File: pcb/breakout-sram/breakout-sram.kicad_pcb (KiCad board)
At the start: 4 copper layers, 62 x 62 mm, 6 parts, among them J1 FX18-120P-0.8SV20, J2 FX18-120S-0.8SV20, U1 IS61WV102416DBLL-10TLI

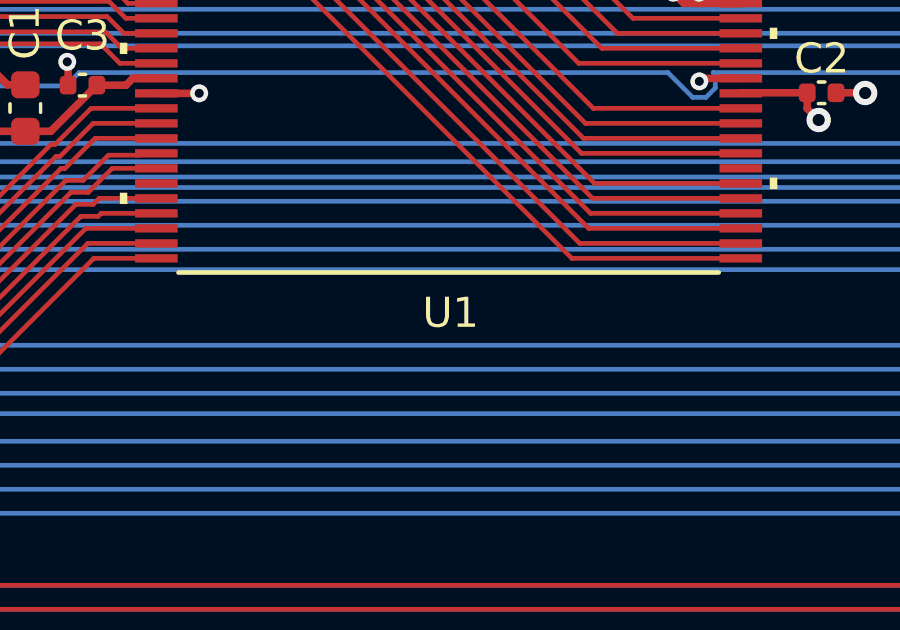
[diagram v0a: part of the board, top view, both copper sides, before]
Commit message: [pcb] misc updates prior to ordder
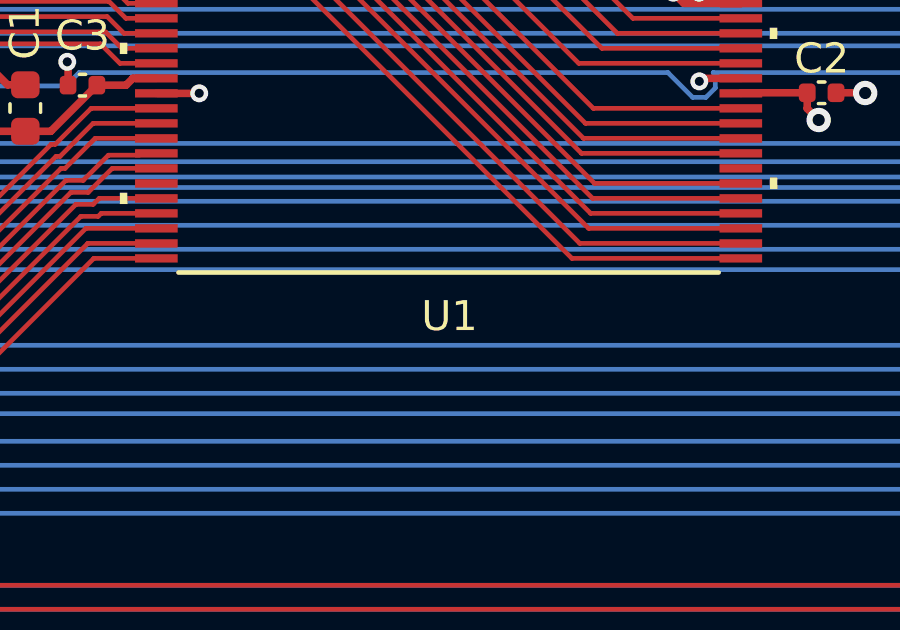
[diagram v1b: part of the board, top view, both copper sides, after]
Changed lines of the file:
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@@
 		(tags "capacitor")
 		(property "Reference" "C1"
-			(at 2.521 -0.014 270)
+			(at 2.521 -0.014 -90)
 			(layer "F.SilkS")
 			(effects
@@
 		)
 		(property "Value" "22uf"
-			(at 0 1.43 270)
+			(at 0 1.43 -90)
 			(layer "F.Fab")
 			(effects
@@
 		)
 		(fp_text user "${REFERENCE}"
-			(at 0 0 270)
+			(at 0 0 -90)
 			(layer "F.Fab")
 			(effects
@@
 		(sheetname "Root")
 		(sheetfile "breakout-sram.kicad_sch")
-		(attr smd)
+		(attr smd dnp)
 		(fp_circle
 			(center -26.701 -3.02)
@@
 		(sheetname "Root")
 		(sheetfile "breakout-sram.kicad_sch")
-		(attr smd)
+		(attr smd dnp)
 		(fp_circle
 			(center -26.701 -3.02)
@@
 		(tags "capacitor")
 		(property "Reference" "C2"
-			(at 0 -1.143 360)
+			(at 0 -1.143 0)
 			(layer "F.SilkS")
 			(effects
@@
 		)
 		(property "Value" "0.1uf"
-			(at 0 1.16 360)
+			(at 0 1.16 0)
 			(layer "F.Fab")
 			(effects
@@
 		)
 		(fp_text user "${REFERENCE}"
-			(at 0 0 360)
+			(at 0 0 0)
 			(layer "F.Fab")
 			(effects
@@
 		(tags "IS61WV102416DBLL-10TLI ")
 		(property "Reference" "U1"
-			(at 0.067 7.568552 0)
+			(at 0.027 7.678552 0)
 			(unlocked yes)
 			(layer "F.SilkS")
@@
 			)
 		)
-		(property "Footprint" "IS61WV102416DBLLIS61WV102416DBLL:IS61WV102416DBLL-10TLI_ISI"
+		(property "Footprint" "IS61WV102416DBLL-10TLI_ISI"
 			(at 0 0 0)
 			(unlocked yes)
@@
 			)
 		)
+		(property "LCSC Part #" " C1348726"
+			(at 0 0 0)
+			(unlocked yes)
+			(layer "F.Fab")
+			(hide yes)
+			(effects
+				(font
+					(size 1 1)
+					(thickness 0.15)
+				)
+			)
+		)
 		(property ki_fp_filters "IS61WV102416DBLL-10TLI_ISI IS61WV102416DBLL-10TLI_ISI-M IS61WV102416DBLL-10TLI_ISI-L")
 		(sheetname "Root")
@@
 		(fp_text user "*"
 			(at -8.9154 -6.0198 0)
+			(unlocked yes)
 			(layer "F.Fab")
 			(effects
